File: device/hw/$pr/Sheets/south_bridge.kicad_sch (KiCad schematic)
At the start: 0 parts

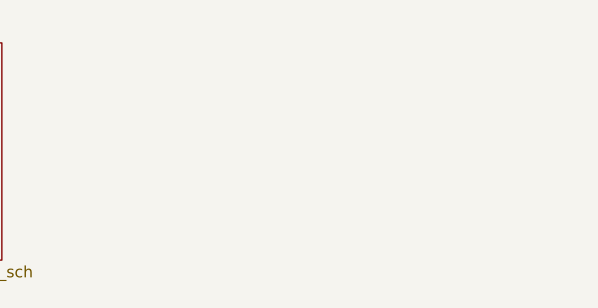
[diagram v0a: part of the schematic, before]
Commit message: New-Sheet
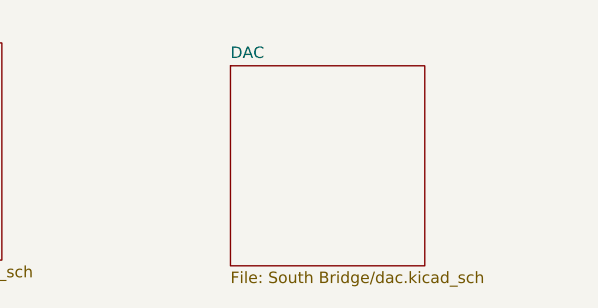
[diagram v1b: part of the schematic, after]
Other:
- added sheet DAC (South Bridge/dac.kicad_sch)
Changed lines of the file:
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@@
+	)
+	(sheet
+		(at 186.69 57.15)
+		(size 21.59 22.225)
+		(fields_autoplaced yes)
+		(stroke
+			(width 0.1524)
+			(type solid)
+		)
+		(fill
+			(color 0 0 0 0.0000)
+		)
+		(property "Sheetname" "DAC"
+			(at 186.69 56.4384 0)
+			(effects
+				(font
+					(size 1.27 1.27)
+				)
+				(justify left bottom)
+			)
+		)
+		(property "Sheetfile" "South Bridge/dac.kicad_sch"
+			(at 186.69 79.9596 0)
+			(effects
+				(font
+					(size 1.27 1.27)
+				)
+				(justify left top)
+			)
+		)
+		(instances
+			(project "medmentum"
+				(path "/ead52261-b3da-41ef-908f-3daaabe10954/940ef1bd-73e9-475b-b1ba-056ab9b45d18"
+					(page "13")
+				)
+			)
+		)
 	)
 	(sheet

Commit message: *
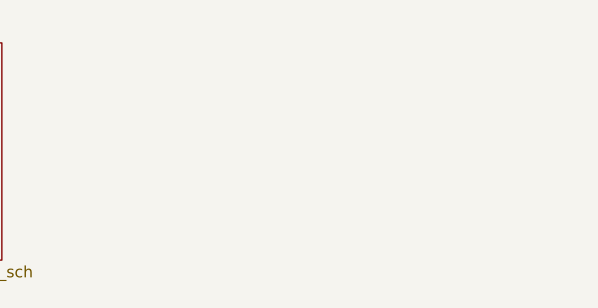
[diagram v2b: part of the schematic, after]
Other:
- removed sheet DAC
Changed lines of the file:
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@@
-	)
-	(sheet
-		(at 186.69 57.15)
-		(size 21.59 22.225)
-		(fields_autoplaced yes)
-		(stroke
-			(width 0.1524)
-			(type solid)
-		)
-		(fill
-			(color 0 0 0 0.0000)
-		)
-		(property "Sheetname" "DAC"
-			(at 186.69 56.4384 0)
-			(effects
-				(font
-					(size 1.27 1.27)
-				)
-				(justify left bottom)
-			)
-		)
-		(property "Sheetfile" "South Bridge/dac.kicad_sch"
-			(at 186.69 79.9596 0)
-			(effects
-				(font
-					(size 1.27 1.27)
-				)
-				(justify left top)
-			)
-		)
-		(instances
-			(project "medmentum"
-				(path "/ead52261-b3da-41ef-908f-3daaabe10954/940ef1bd-73e9-475b-b1ba-056ab9b45d18"
-					(page "13")
-				)
-			)
-		)
 	)
 	(sheet
